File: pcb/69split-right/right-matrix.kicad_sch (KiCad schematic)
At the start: 78 parts, among them SW1 &,7,,F7, SW10 I, SW11 O, SW12 P, SW13 {,[, SW14 },], SW15 Enter, SW16 Delete,Insert, SW17 H, SW18 J, SW19 K, SW2 *,8,,F8, SW20 L, SW21 :,;, SW22 @,', SW23 #,~, SW24 Home,PgUp, SW25 N, SW26 M, SW27 <,,, SW28 >,., SW29 ?,/, SW3 (,9,,F9, SW30 Shift, SW31 ↑, SW32 End,PgDn, SW33 Space, SW34 Alt,`,¬, SW35 Fn, SW36 Ctrl, SW37 ←, SW38 ↓, SW39 →, SW4 ),0,,F10, SW5 _,-,,F11, SW6 +,=,,F12, SW7 Backspace, SW8 Y, SW9 U

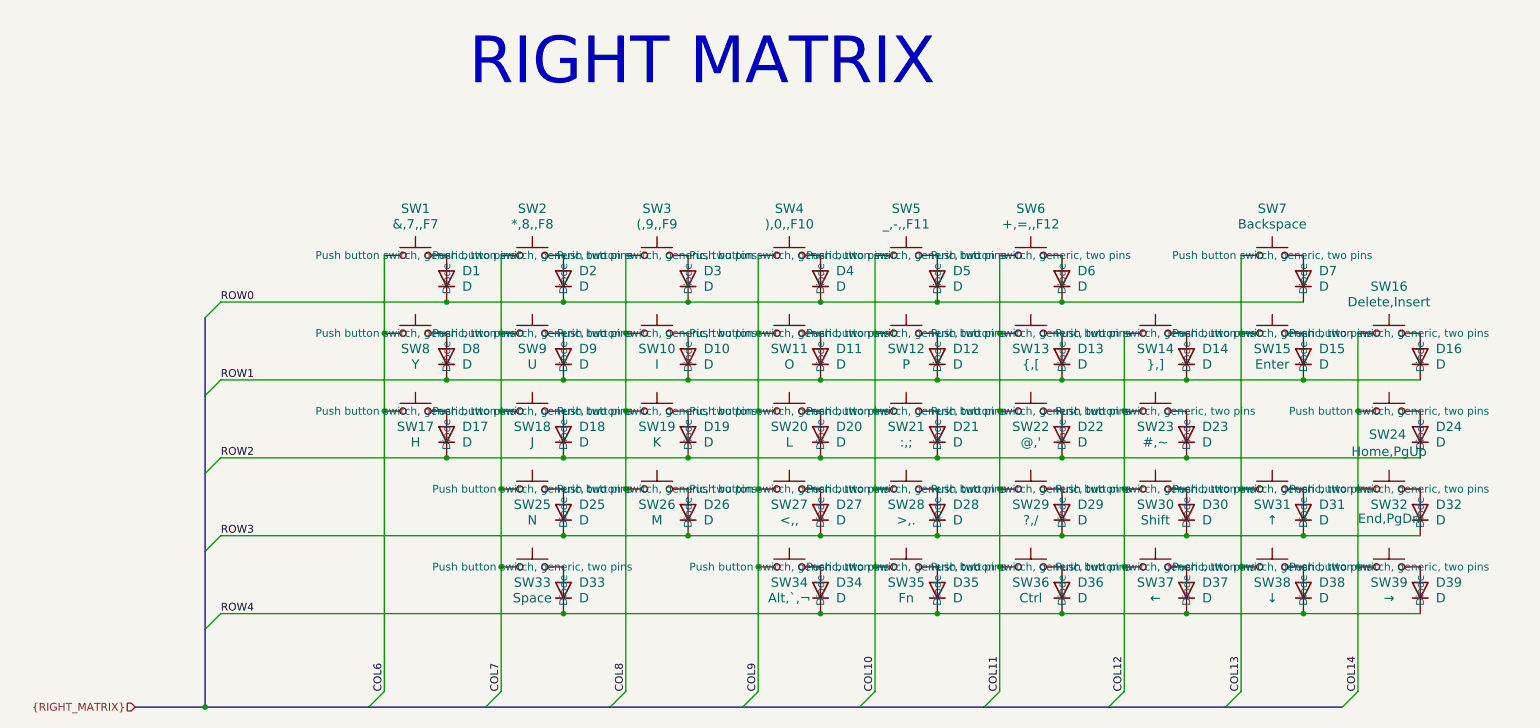
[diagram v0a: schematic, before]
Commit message: Alright I think now the left side is actually ready.
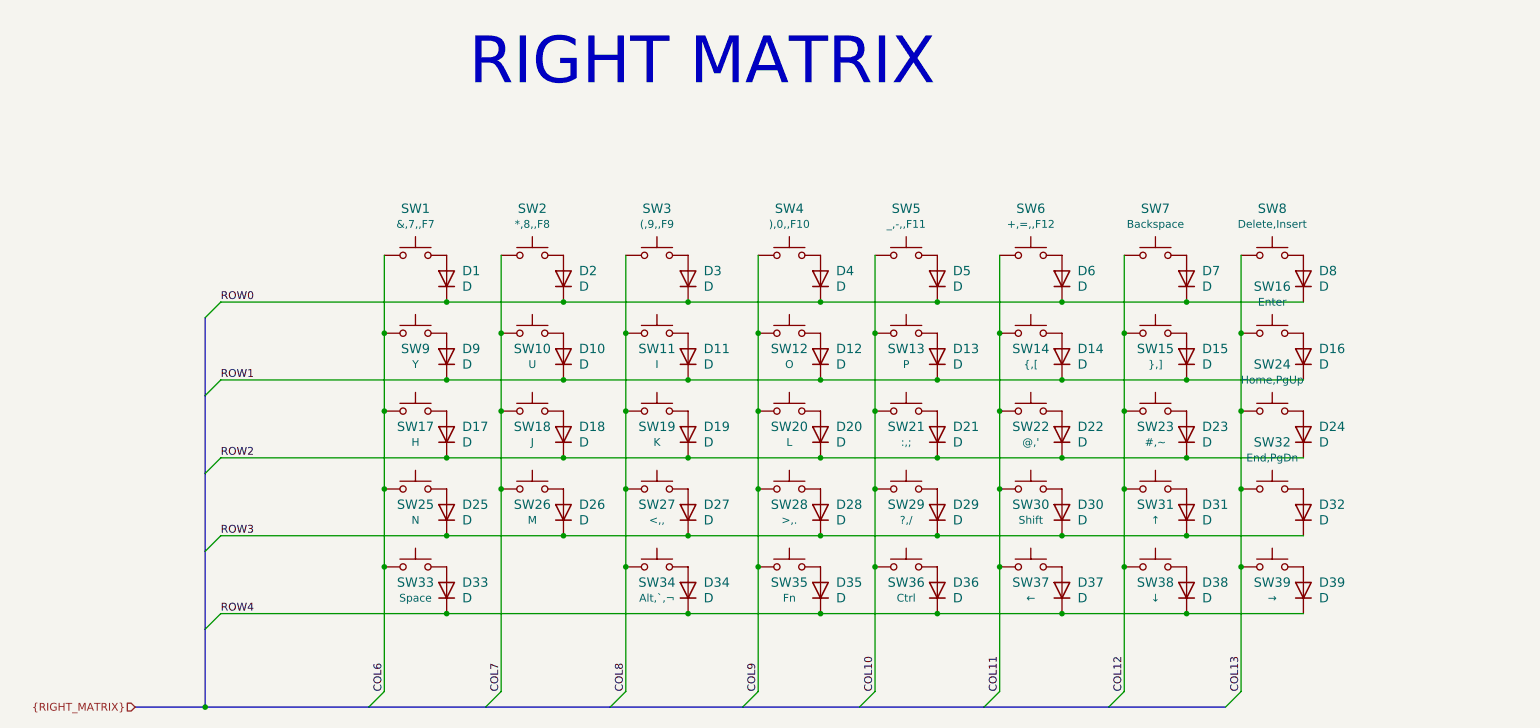
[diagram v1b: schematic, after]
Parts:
- SW1: value &,7,,F7 -> SW_Push; Key (none) -> &,7,,F7
- SW10: renamed from SW9; value U -> SW_Push; Key (none) -> U
- SW11: renamed from SW10; value I -> SW_Push; Key (none) -> I
- SW12: renamed from SW11; value O -> SW_Push; Key (none) -> O
- SW13: renamed from SW12; value P -> SW_Push; Key (none) -> P
- SW14: renamed from SW13; value {,[ -> SW_Push; Key (none) -> {,[
- SW15: renamed from SW14; value },] -> SW_Push; Key (none) -> },]
- SW16: renamed from SW15; value Enter -> SW_Push; Key (none) -> Enter
- SW17: value H -> SW_Push; Key (none) -> H
- SW18: value J -> SW_Push; Key (none) -> J
- SW19: value K -> SW_Push; Key (none) -> K
- SW2: value *,8,,F8 -> SW_Push; Key (none) -> *,8,,F8
- SW20: value L -> SW_Push; Key (none) -> L
- SW21: value :,; -> SW_Push; Key (none) -> :,;
- SW22: value @,' -> SW_Push; Key (none) -> @,'
- SW23: value #,~ -> SW_Push; Key (none) -> #,~
- SW24: value Home,PgUp -> SW_Push; Key (none) -> Home,PgUp
- SW25: value N -> SW_Push; Key (none) -> N
- SW26: value M -> SW_Push; Key (none) -> M
- SW27: value <,, -> SW_Push; Key (none) -> <,,
- SW28: value >,. -> SW_Push; Key (none) -> >,.
- SW29: value ?,/ -> SW_Push; Key (none) -> ?,/
- SW3: value (,9,,F9 -> SW_Push; Key (none) -> (,9,,F9
- SW30: value Shift -> SW_Push; Key (none) -> Shift
- SW31: value ↑ -> SW_Push; Key (none) -> ↑
- SW32: value End,PgDn -> SW_Push; Key (none) -> End,PgDn
- SW33: value Space -> SW_Push; Key (none) -> Space
- SW34: value Alt,`,¬ -> SW_Push; Key (none) -> Alt,`,¬
- SW35: value Fn -> SW_Push; Key (none) -> Fn
- SW36: value Ctrl -> SW_Push; Key (none) -> Ctrl
- SW37: value ← -> SW_Push; Key (none) -> ←
- SW38: value ↓ -> SW_Push; Key (none) -> ↓
- SW39: value → -> SW_Push; Key (none) -> →
- SW4: value ),0,,F10 -> SW_Push; Key (none) -> ),0,,F10
- SW5: value _,-,,F11 -> SW_Push; Key (none) -> _,-,,F11
- SW6: value +,=,,F12 -> SW_Push; Key (none) -> +,=,,F12
- SW7: value Backspace -> SW_Push; Key (none) -> Backspace
- SW8: renamed from SW16; value Delete,Insert -> SW_Push; Key (none) -> Delete,Insert
- SW9: renamed from SW8; value Y -> SW_Push; Key (none) -> Y
- renumbered D9 to D10, D10 to D11, D11 to D12, D12 to D13, D13 to D14, D14 to D15, D15 to D16, D16 to D8, D8 to D9
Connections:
- net COL14 is gone; now on net COL13: SW24.1, SW32.1, SW39.1, SW8.1
- net COL10: now also SW29.1, SW36.1; no longer SW28.1, SW35.1
- net COL11: now also SW30.1, SW37.1; no longer SW29.1, SW36.1
- net COL12: now also SW31.1, SW38.1, SW7.1; no longer SW30.1, SW37.1
- net COL13: no longer SW31.1, SW38.1, SW7.1
- net COL6: now also SW25.1, SW33.1
- net COL7: now also SW26.1; no longer SW25.1, SW33.1
- net COL8: now also SW27.1, SW34.1; no longer SW26.1
- net COL9: now also SW28.1, SW35.1; no longer SW27.1, SW34.1
- net ROW0: now also D8.1 (K)
- net ROW1: no longer D8.1 (K)
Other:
- moved on the sheet: D24, D25, D26, D27, D28, D29, D30, D31, D32, D33, D34, D35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
